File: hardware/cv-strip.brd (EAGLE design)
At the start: 152.5 x 43.6 mm, 83 parts, among them IC1 PIC16F1825SO14, IC2 74HC595D, IC3 74HC595D, IC4 MCP4728_QUAD_DAC, IC5 LM324D, IC6 REG1117, IC7 6N138

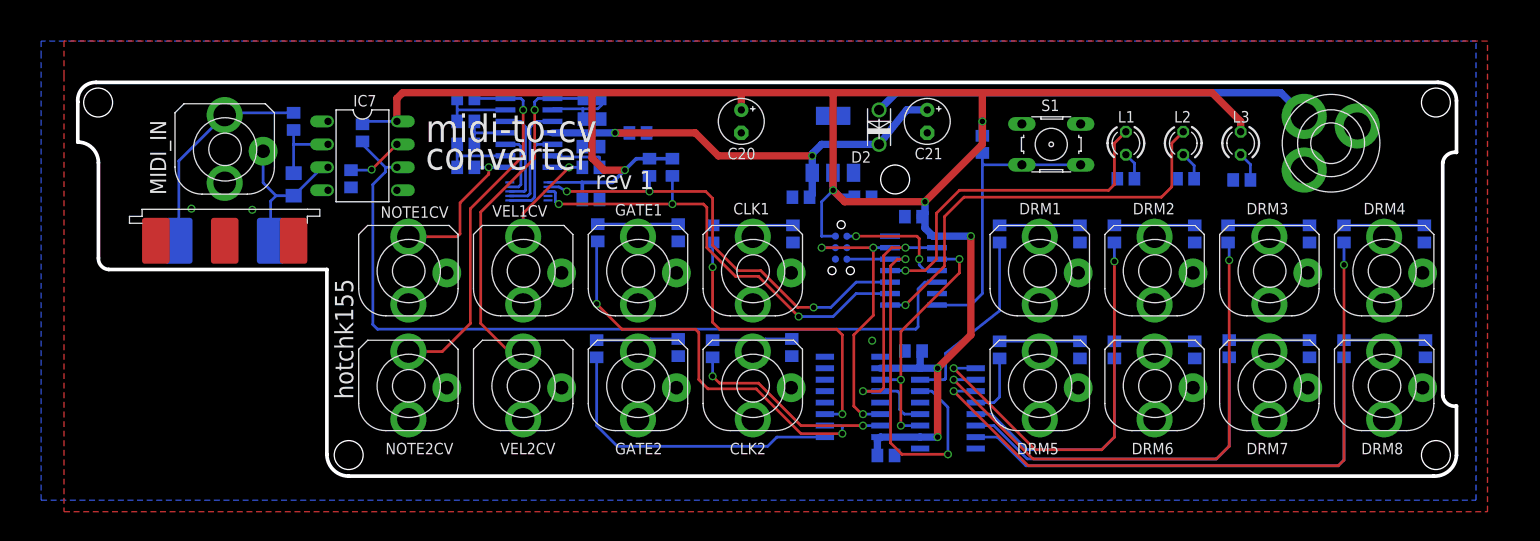
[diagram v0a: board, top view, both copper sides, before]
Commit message: rev2 updates - checking needed
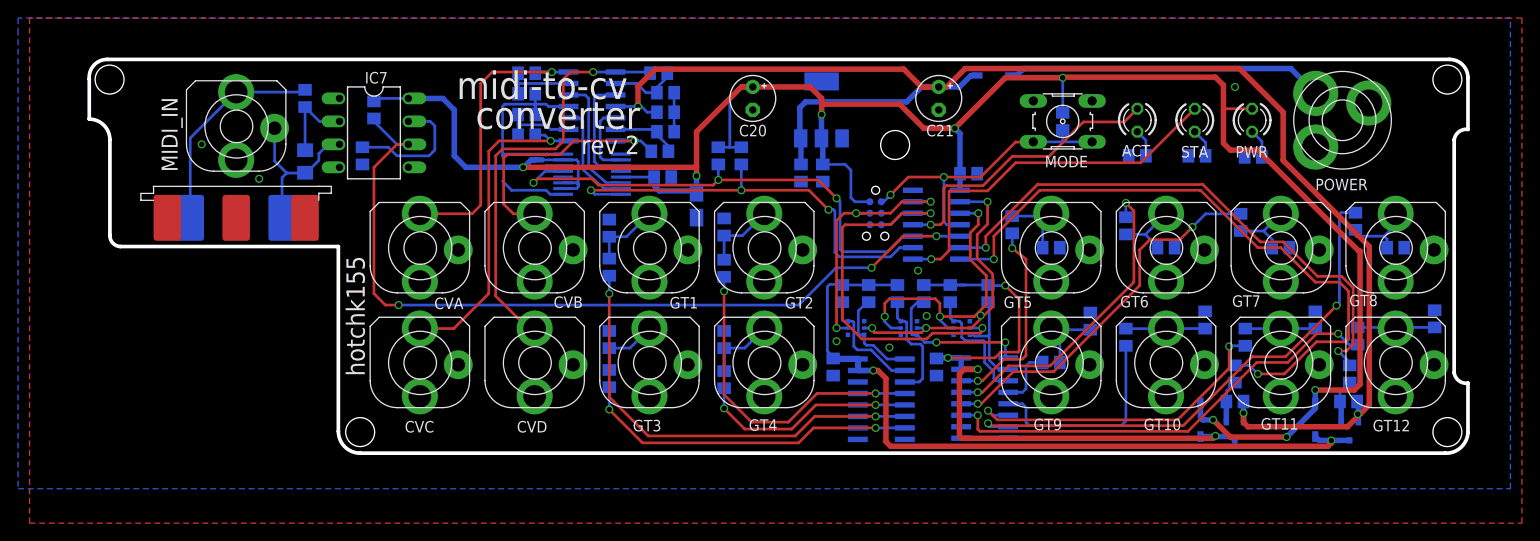
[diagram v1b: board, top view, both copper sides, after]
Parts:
- removed CLK1, CLK2, DRM1, DRM2, DRM3, DRM4, DRM5, DRM6, DRM7, DRM8, GATE1, GATE2, NOTE1CV, NOTE2CV, VEL1CV, VEL2CV: VERTICAL_3_5MM_SOCKET, jason_eagle6:VERTICAL_3_5MM_SOCKET
- removed D2: 1N4004, jasons_stuff:DO-VERT
- removed L1, L2, L3: (no value), led:LED3MM
- removed S1: (no value), switch-omron:B3F-10XX
- added ACT, PWR, STA: (no value), led:LED3MM
- added C22: (no value), microbuilder:EIA3216-18/A-R
- added CVA, CVB, CVC, CVD, GT1, GT10, GT11, GT12, GT2, GT3, GT4, GT5, GT6, GT7, GT8, GT9: VERTICAL_3_5MM_SOCKET, jason_eagle6:VERTICAL_3_5MM_SOCKET
- added D3, D4, D5: (no value), microbuilder:SOD-123
- added MODE: (no value), switch-omron:B3F-10XX
- added Q1, Q2, Q4: (no value), microbuilder:SOT363
- added Q3, Q5: (no value), microbuilder:SOT23-R
- added R30, R31, R32, R33, R34, R35, R36, R37, R38, R39: (no value), rcl:R0805
- IC2: value 74HC595D -> AD5696R; device 74xx-eu:SO16 -> jason_eagle6:SSOP16
- IC3: value 74HC595D -> MC14094B; device 74xx-eu:SO16 -> jason_eagle6:SO16
- IC4: value MCP4728_QUAD_DAC -> MC14094B; device jason_eagle6:MSOP10 -> jason_eagle6:SO16
- moved IC4 55.4 mm to (100.6, 7.49)
- moved IC2 47.1 mm to (57.1, 32.3)
- moved R8 15.3 mm to (108.0, 11.4), turned to 180 degrees
- moved R10 14.0 mm to (128.9, 26.9), turned to 270 degrees
- moved R12 13.9 mm to (103.6, 26.7)
- moved R11 13.8 mm to (116.2, 26.5), turned to 270 degrees
- moved C7 11.7 mm to (120.7, 24.1), turned to 180 degrees
- moved C8 11.7 mm to (108.0, 24.1), turned to 180 degrees
- moved C6 11.6 mm to (133.3, 24.1), turned to 180 degrees
- moved R6 11.6 mm to (129.4, 14.2)
- moved R7 11.5 mm to (116.2, 14.2)
- moved C13 11.4 mm to (83.8, 10.9), turned to 270 degrees
- moved C4 9.72 mm to (112.3, 16.0), turned to 90 degrees
- moved C3 9.59 mm to (125.0, 16.1), turned to 90 degrees
- moved C2 9.55 mm to (137.2, 16.1), turned to 90 degrees
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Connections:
- removed net MIDI_OUT: IC1.6
- removed net N$22: IC1.9, IC4.3, R21.2
- removed net N$47: IC2.3, R5.1
- removed net N$51: IC2.4, R12.1
- removed net N$53: IC2.7, R9.1
- new net GT1_VSEL: IC1.6, R38.1
- new net GT2_VSEL: IC1.7, R39.1
- new net N$10: IC3.5, R15.1
- new net N$11: IC3.7, R16.1
- new net N$14: IC3.1, Q1.3, R31.1
- new net N$17: IC4.11, R9.1
- new net N$18: IC4.12, R10.1
- new net N$19: IC4.13, R11.1
- new net N$38: IC4.14, R12.1
- new net N$44: IC4.6, R6.1
- new net N$45: IC4.5, R7.1
- new net SCL: IC1.10, IC2.P$13, R22.2
- new net SDA: IC1.9, IC2.P$8, R21.2
- new net VDD_GT1: C13.1, D3.C, IC3.15, IC3.16, Q3.3, R30.2, R31.2, R32.2
- new net VDD_GT2: C12.1, D4.C, IC4.15, IC4.16, Q5.3, R33.2, R34.2, R35.2
- net ACT_LED: now also ACT.A; no longer L1.A
- net GND: now also C22.-, C9.2, CVA.2, CVB.2, CVC.2, CVD.2, GT1.2, GT10.2, GT11.2, GT12.2, GT2.2, GT3.2, GT4.2, GT5.2, GT6.2, GT7.2, GT8.2, GT9.2, IC2.P$12, IC2.P$14, IC2.P$16, IC2.P$4, IC2.P$9, IC4.8, MODE.3, MODE.4, Q1.1, Q1.4, Q2.1, Q2.4, Q4.1, Q4.4; no longer C9.1, CLK1.2, CLK2.2, DRM1.2, DRM2.2, DRM3.2, DRM4.2, DRM5.2, DRM6.2, DRM7.2, DRM8.2, GATE1.2, GATE2.2, IC2.13, IC2.8, IC3.13, IC4.10, IC4.4, NOTE1CV.2, NOTE2CV.2, S1.3, S1.4, VEL1CV.2, VEL2CV.2
- net N$1: now also GT4.4; no longer CLK2.4
- net N$12: now also IC3.6, R14.1; no longer IC3.15, R15.1
- net N$13: now also IC3.4, R13.1; no longer IC3.1, R16.1
- net N$15: now also IC3.2, Q1.6, R30.1; no longer IC3.3, R13.1
- net N$16: now also IC3.3, Q2.6, R32.1; no longer IC3.2, R14.1
- net N$2: now also CVD.4; no longer VEL2CV.4
- net N$20: now also GT9.4; no longer DRM1.4
- net N$21: now also Q5.1, R37.1, R39.2; no longer IC1.10, IC4.2, R22.2
- net N$23: now also GT10.4; no longer DRM2.4
- net N$24: now also GT11.4; no longer DRM3.4
- net N$3: now also CVB.4; no longer VEL1CV.4
- net N$32: now also GT8.4; no longer DRM4.4
- net N$33: now also GT5.4; no longer DRM5.4
- net N$34: now also MODE.1, MODE.2, R4.2
- net N$35: now also PWR.K; no longer L3.K
- net N$36: now also ACT.K; no longer L1.K
- net N$37: now also STA.K; no longer L2.K
- net N$39: now also GT6.4; no longer DRM6.4
- net N$4: now also CVC.4; no longer NOTE1CV.4
- net N$40: now also D5.A; no longer D2.A
- net N$41: now also GT7.4; no longer DRM7.4
- net N$43: now also IC4.7, R5.1; no longer IC2.15, R8.1
- net N$46: now also IC4.4, R8.1; no longer IC2.1, R7.1
- net N$48: now also IC4.1, Q2.3, R33.1; no longer IC2.2, R6.1
- net N$49: now also IC4.2, Q4.3, R34.1; no longer IC2.5, R11.1
- net N$5: now also CVA.4; no longer NOTE2CV.4
- net N$50: now also IC4.3, Q4.6, R35.1; no longer IC2.6, R10.1
- net N$52: now also GT12.4; no longer DRM8.4
- net N$6: now also GT3.4; no longer GATE2.4
- net N$7: now also GT1.4; no longer GATE1.4
- net N$8: now also GT2.4; no longer CLK1.4
- net N$9: now also Q3.1, R36.1, R38.2; no longer IC1.7, R4.2, S1.1, S1.2
- net SR_CLK: now also Q2.5, Q4.5; no longer IC2.11, IC3.11
- net SR_DAT: now also Q1.5; no longer IC3.14
- net SR_DAT2: now also Q4.2; no longer IC2.14
- net SR_RCK: now also Q1.2, Q2.2; no longer IC2.12, IC3.12
- net STATUS_LED: now also STA.A; no longer L2.A
- net VDD: now also C22.+, C9.1, D3.A, D4.A, IC2.P$10, IC2.P$11, IC2.P$15, IC2.P$5, PWR.A; no longer C12.1, C13.1, C9.2, IC2.10, IC2.16, IC3.10, IC3.16, IC4.1, L3.A
- net VIN: now also D5.C, Q3.2, Q5.2, R36.2, R37.2; no longer D2.C
- net VOUTA: now also IC2.P$3, IC5.3; no longer IC4.6, IC5.5
- net VOUTB: now also IC2.P$2, IC5.5; no longer IC4.7, IC5.3
- net VOUTC: now also IC2.P$6; no longer IC4.8
- net VOUTD: now also IC2.P$7; no longer IC4.9
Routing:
- net VIN: track 51.3 -> 169.3 mm, vias 2 -> 3
- net VDD_GT1: track 0.00 -> 88.5 mm, vias 0 -> 2
- net VDD_GT2: track 0.00 -> 76.0 mm, vias 0 -> 4
- net N$47: track 73.4 -> 0.00 mm, vias 2 -> 0
- net GT2_VSEL: track 0.00 -> 72.1 mm, vias 0 -> 2
- net GT1_VSEL: track 0.00 -> 62.2 mm, vias 0 -> 2
- net SCL: track 0.00 -> 55.3 mm, vias 0 -> 3
- net N$53: track 53.7 -> 0.00 mm
- net N$22: track 50.9 -> 0.00 mm, vias 3 -> 0
- net N$17: track 0.00 -> 50.5 mm, vias 0 -> 2
- net SDA: track 0.00 -> 48.1 mm, vias 0 -> 3
- net N$21: track 49.4 -> 4.79 mm, vias 3 -> 0
- net N$48: track 59.7 -> 17.1 mm
- net N$18: track 0.00 -> 41.9 mm, vias 0 -> 2
- net N$46: track 46.1 -> 6.67 mm, vias 2 -> 0
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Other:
- board text added: "POWER"
- board text added: "rev 2"
- board text removed: "rev 1"
